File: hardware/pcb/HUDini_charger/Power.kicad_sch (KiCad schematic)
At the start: 25 parts, among them J1 USB_C_Receptacle_PowerOnly_6P, Q1 CHG (GDS), Q2 DSG (GDS), U2 LM3671, U3 BQ29700DSER, U4 MCP73831-2-OT

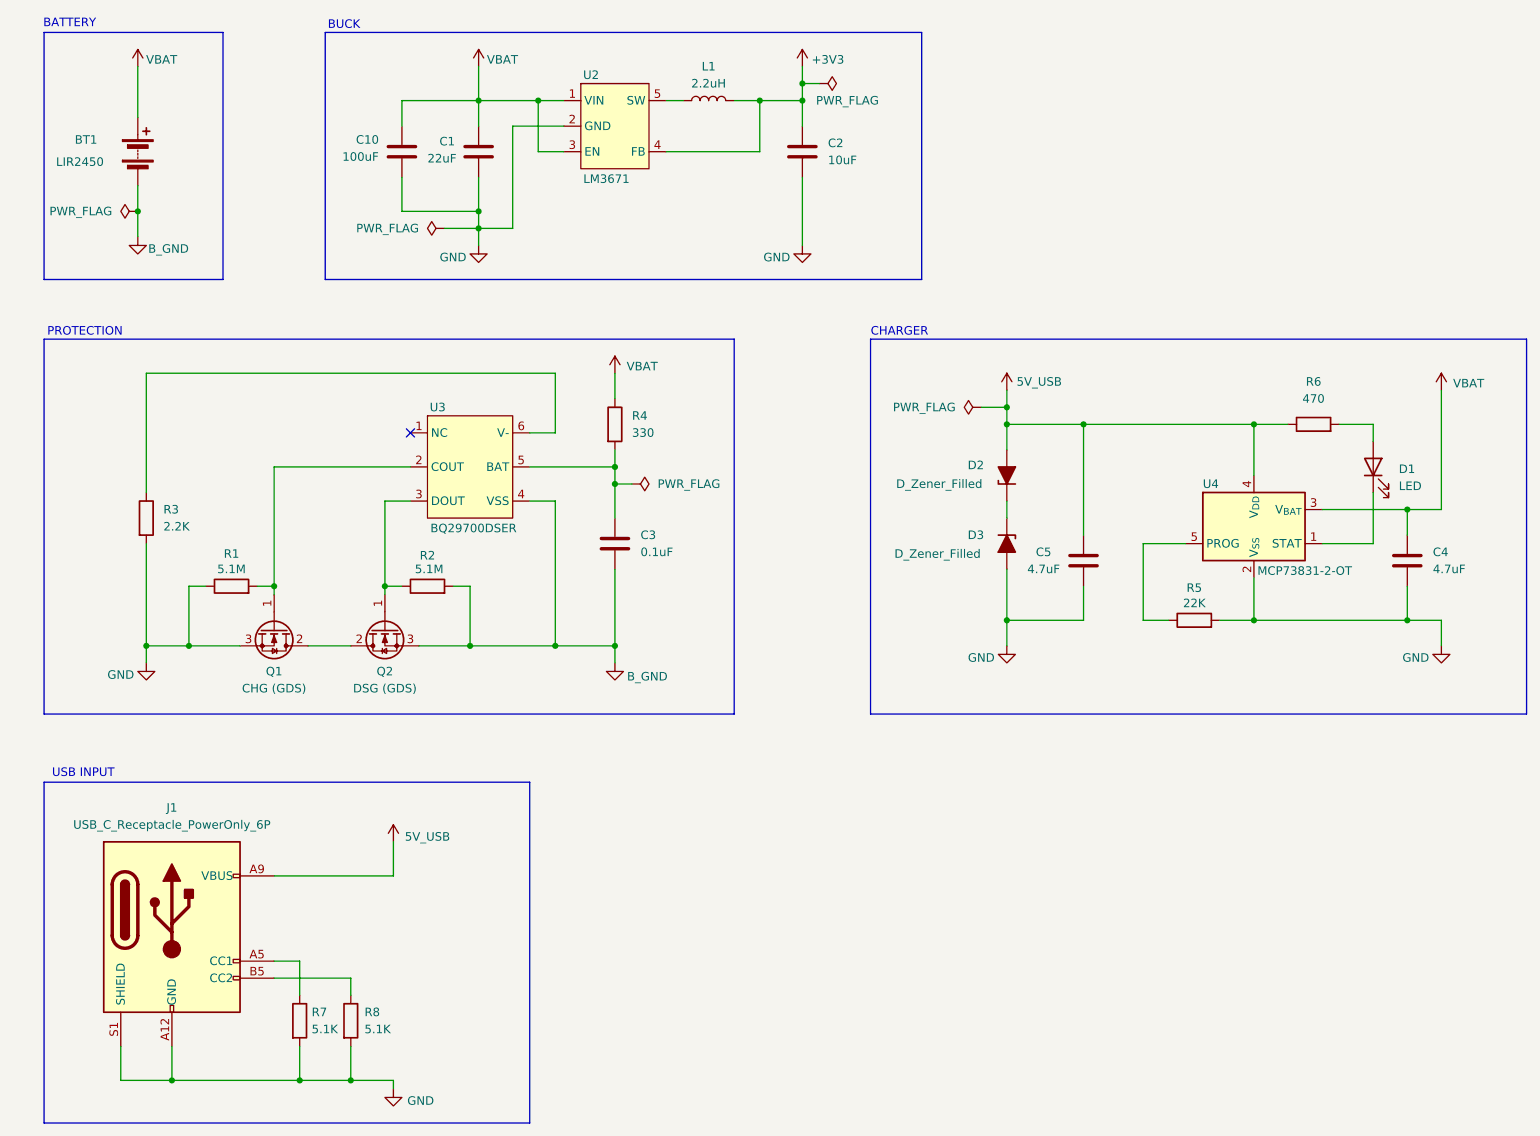
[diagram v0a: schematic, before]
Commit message: Updated PCB Files
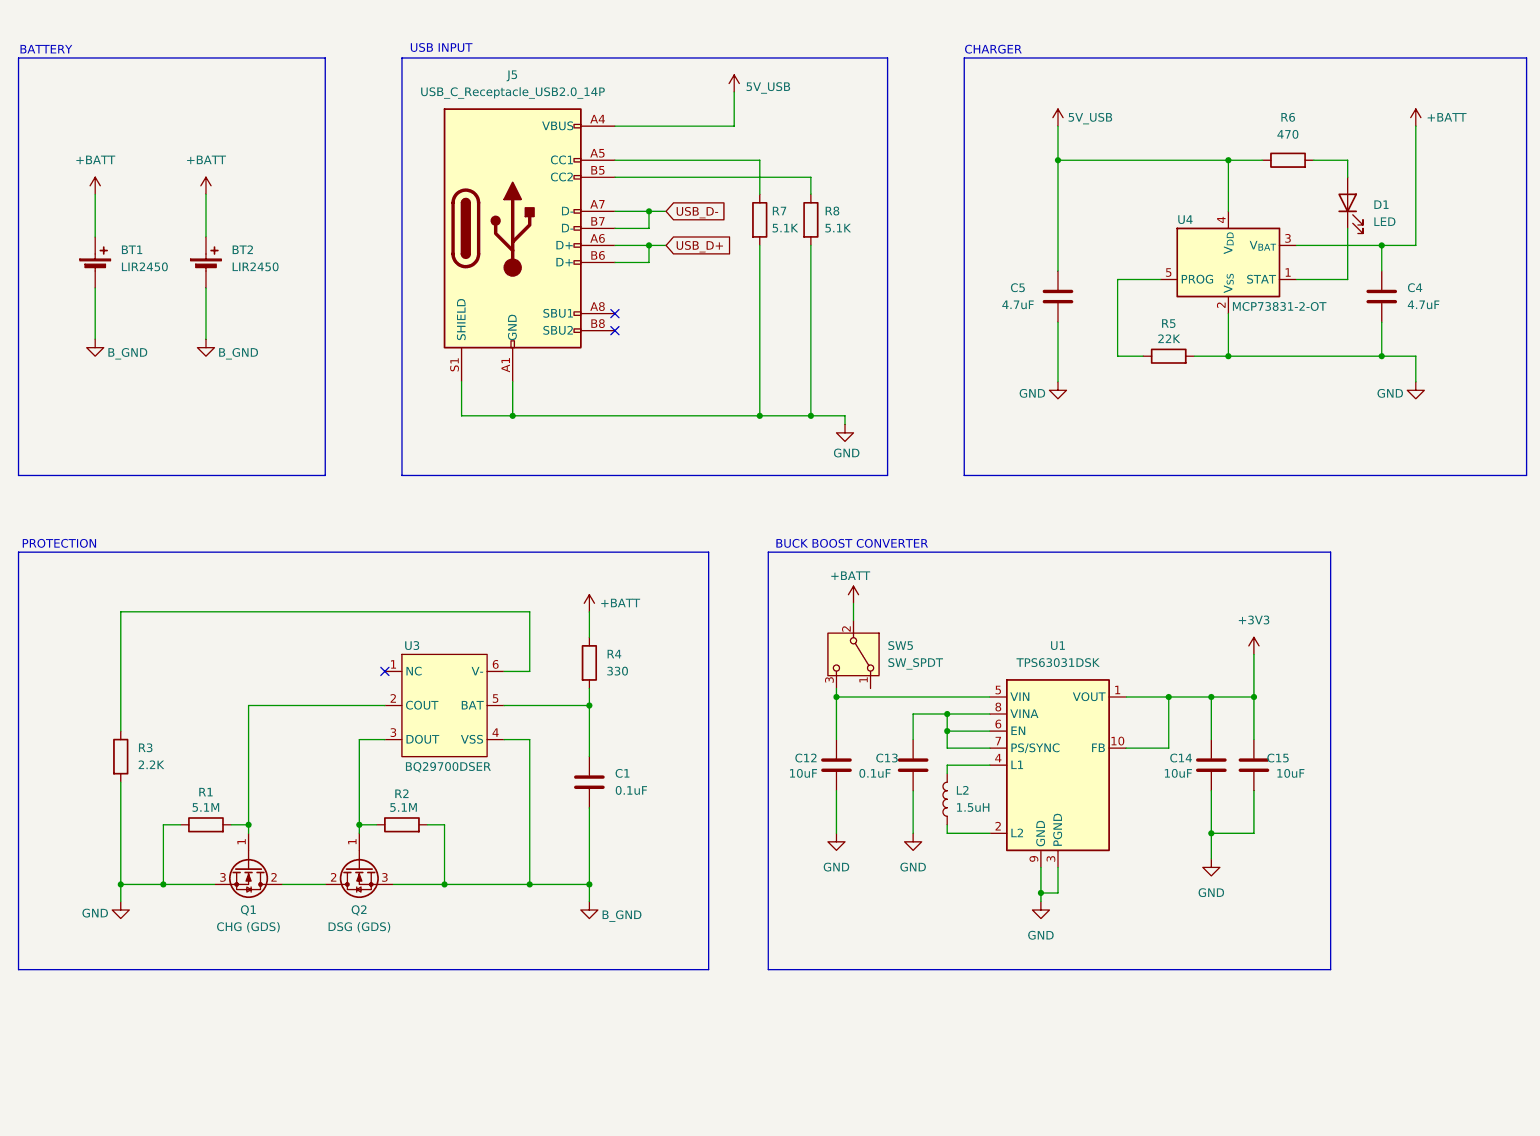
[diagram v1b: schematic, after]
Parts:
- removed BT1: LIR2450, Battery:BatteryHolder_Keystone_3009_1x2450, symbol Device:Battery
- removed C10: 100uF, Capacitor_SMD:C_0603_1608Metric, symbol Device:C
- removed C2: 10uF, Capacitor_SMD:C_0603_1608Metric, symbol Device:C
- removed C3: 0.1uF, Capacitor_SMD:C_0603_1608Metric, symbol Device:C
- removed D2, D3: D_Zener_Filled, Diode_SMD:D_SOD-323, symbol Device:D_Zener_Filled
- removed J1: USB_C_Receptacle_PowerOnly_6P, Connector_USB:USB_C_Receptacle_HRO_TYPE-C-31-M-12, symbol Connector:USB_C_Receptacle_PowerOnly_6P
- removed L1: 2.2uH, Inductor_SMD:L_1210_3225Metric, symbol Device:L
- removed U2: LM3671, Package_TO_SOT_SMD:SOT-23-5, symbol Glasses_Custom_Symbols:LM3671
- added BT1, BT2: LIR2450, Connector_Wire:SolderWire-0.15sqmm_1x02_P4mm_D0.5mm_OD1.5mm, symbol Device:Battery_Cell
- added C12, C14, C15: 10uF, Capacitor_SMD:C_0603_1608Metric_Pad1.08x0.95mm_HandSolder, symbol Device:C
- added C13: 0.1uF, Capacitor_SMD:C_0603_1608Metric_Pad1.08x0.95mm_HandSolder, symbol Device:C
- added J5: USB_C_Receptacle_USB2.0_14P, Connector_USB:USB_C_Receptacle_GCT_USB4085, symbol Connector:USB_C_Receptacle_USB2.0_16P
- added L2: 1.5uH, Inductor_SMD:L_0603_1608Metric_Pad1.05x0.95mm_HandSolder, symbol Device:L
- added SW5: SW_SPDT, Button_Switch_THT:SW_E-Switch_EG1224_SPDT_Angled, symbol Switch:SW_SPDT
- added U1: TPS63031DSK, Package_SON:WSON-10-1EP_2.5x2.5mm_P0.5mm_EP1.2x2mm, symbol Regulator_Switching:TPS63031DSK
- C1: value 22uF -> 0.1uF; footprint Capacitor_SMD:C_0603_1608Metric -> Capacitor_SMD:C_0603_1608Metric_Pad1.08x0.95mm_HandSolder
- R1: footprint Resistor_SMD:R_0603_1608Metric -> Resistor_SMD:R_0603_1608Metric_Pad0.98x0.95mm_HandSolder; now left out of the parts list
- R2, R3, R4: footprint Resistor_SMD:R_0603_1608Metric -> Resistor_SMD:R_0603_1608Metric_Pad0.98x0.95mm_HandSolder
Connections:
- net +3V3: now also C14.1, C15.1, U1.1 (VOUT), U1.10 (FB)
- net 5V_USB: now also J5.A4 (VBUS), J5.A9 (VBUS), J5.B4 (VBUS), J5.B9 (VBUS)
- net B_GND: now also C1.2, BT1.2 (-), BT2.2 (-)
- net GND: now also C12.2, C13.1, C14.2, C15.2, J5.A1 (GND), J5.A12 (GND), J5.B1 (GND), J5.B12 (GND), J5.S1 (SHIELD), U1.11 (PGND), U1.3 (PGND), U1.9 (GND); no longer C1.2
- net at R7.1: now also J5.A5 (CC1)
- net at R4.2, U3.5 (BAT): now also C1.1
- net at R8.1: now also J5.B5 (CC2)
- net VBAT renamed +BATT
- net +BATT: now also BT1.1 (+), BT2.1 (+), SW5.2 (B); no longer C1.1
- new net: L2.1, U1.2 (L2)
- new net: L2.2, U1.4 (L1)
- new net: C13.2, U1.6 (EN), U1.7 (PS/SYNC), U1.8 (VINA)
- new net: C12.1, SW5.3 (C), U1.5 (VIN)
- new net USB_D+: J5.A6 (D+), J5.B6 (D+)
- new net USB_D-: J5.A7 (D-), J5.B7 (D-)
- no-connect marks 1 -> 3
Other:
- note added: "BUCK BOOST CONVERTER"
- note removed: "BUCK"
- moved on the sheet: C4, C5, D1, Q1, Q2, R1, R2, R3, R4, R5, R6, R7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
